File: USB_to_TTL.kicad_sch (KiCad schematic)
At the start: 3 parts, among them J501 USB_B_Mini, U501 CH340C

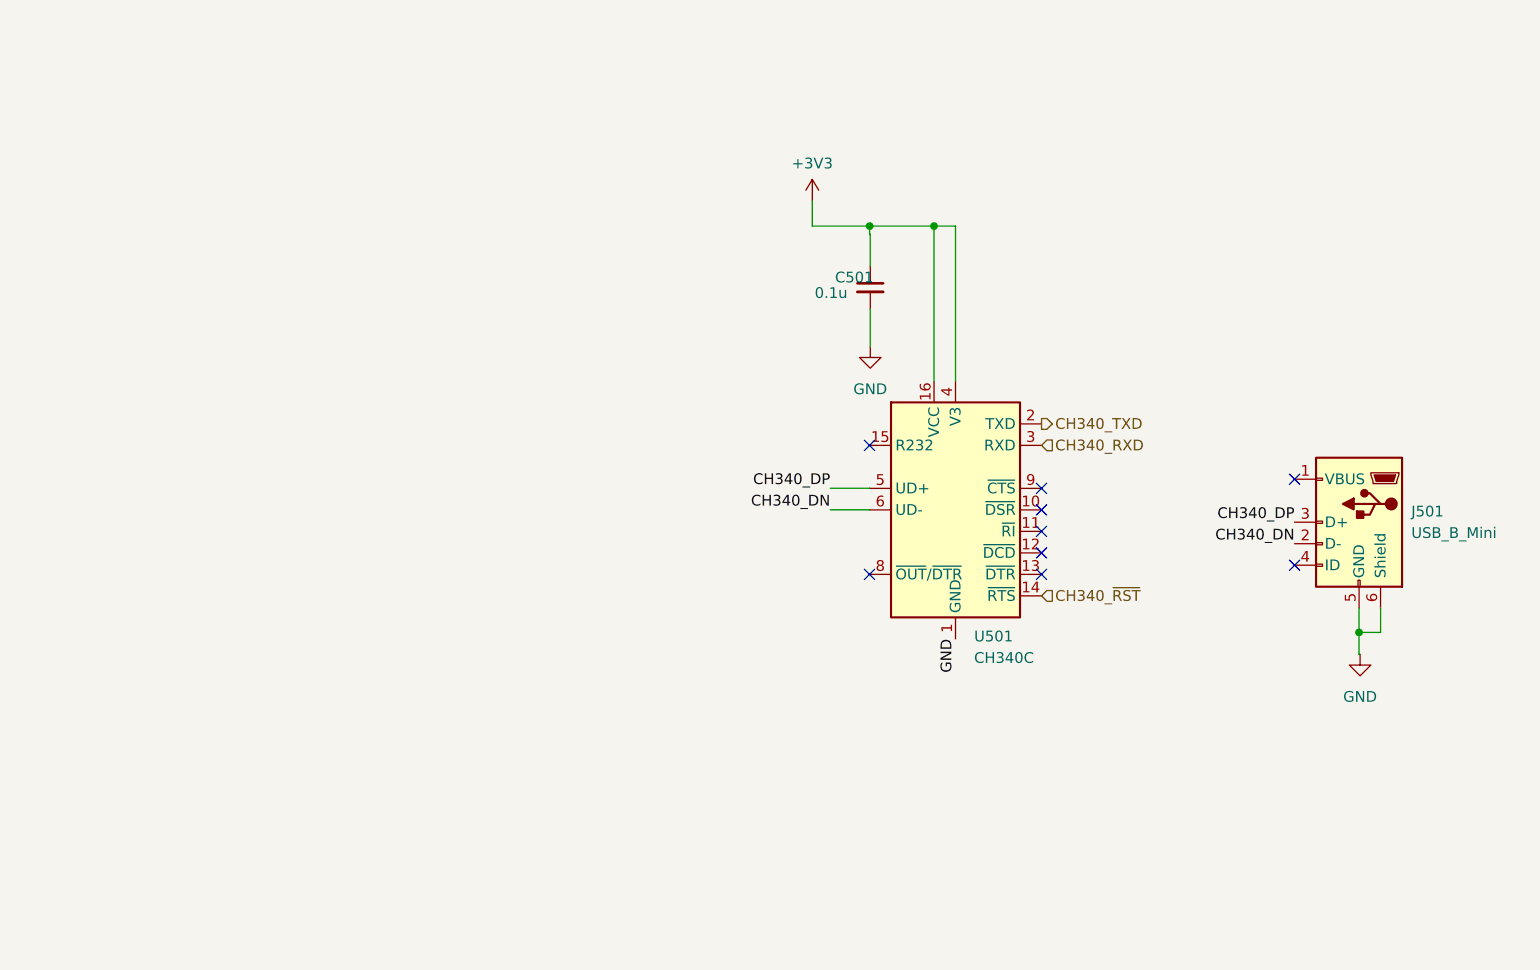
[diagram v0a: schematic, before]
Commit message: schematic pages are reviewed
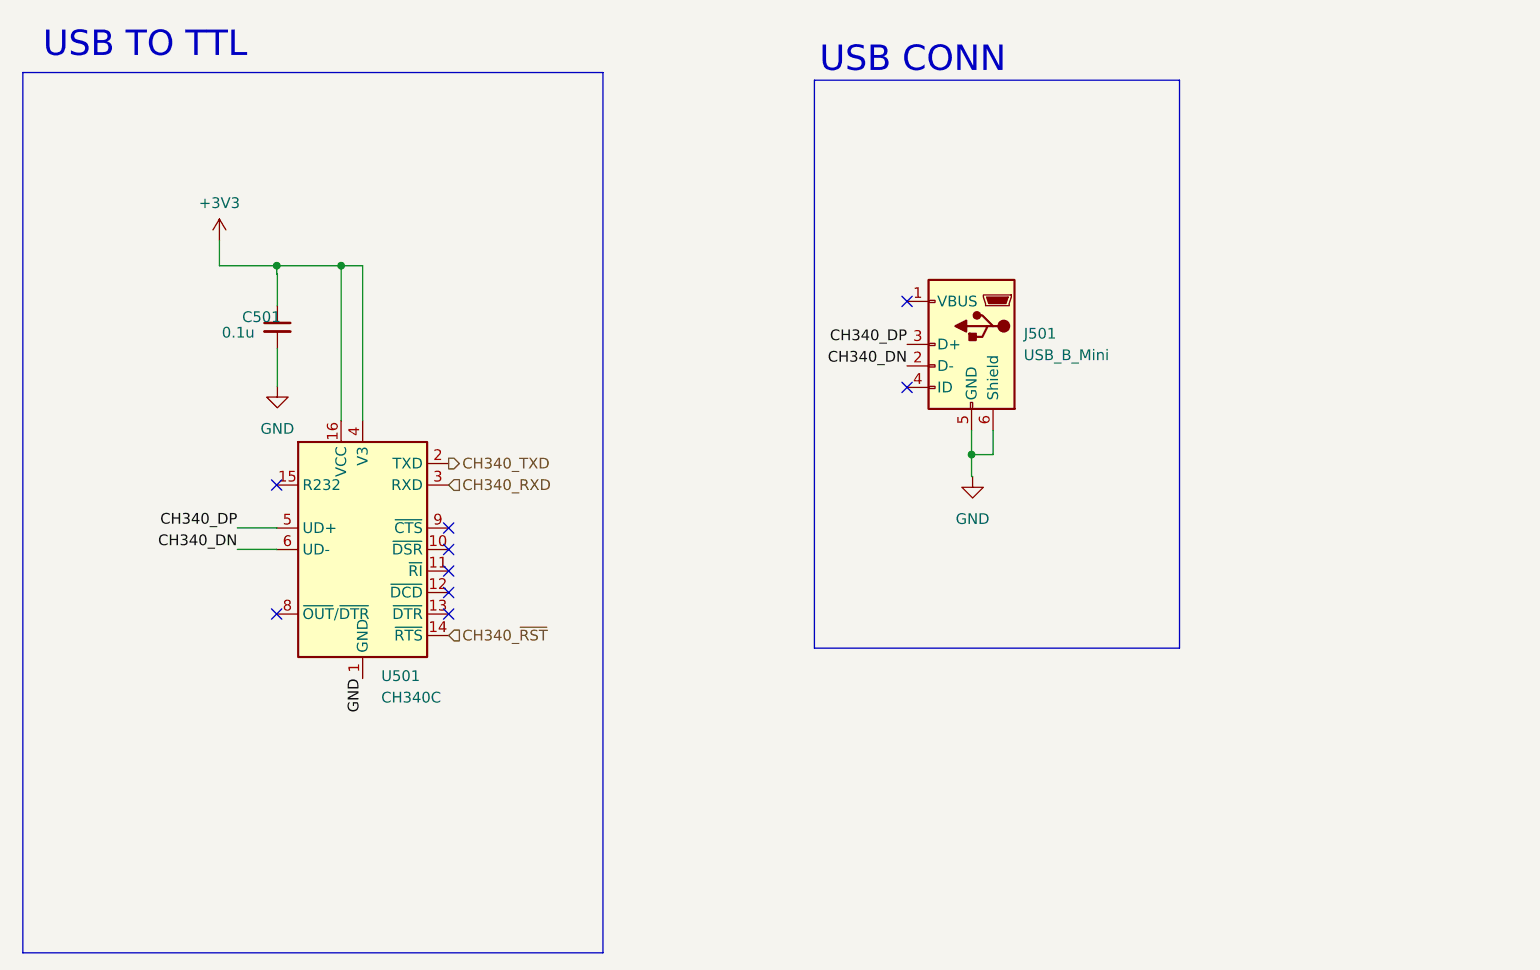
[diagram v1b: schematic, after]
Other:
- note added: "USB CONN"
- note added: "USB TO TTL"
- moved on the sheet: C501, J501, U501
